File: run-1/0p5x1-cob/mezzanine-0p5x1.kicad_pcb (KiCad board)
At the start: 2 copper layers, 14 x 16 mm, 11 parts

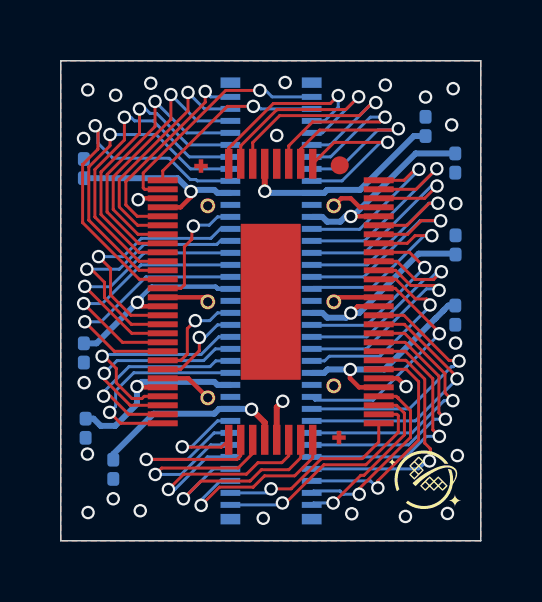
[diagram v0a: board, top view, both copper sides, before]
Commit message: Tweaks
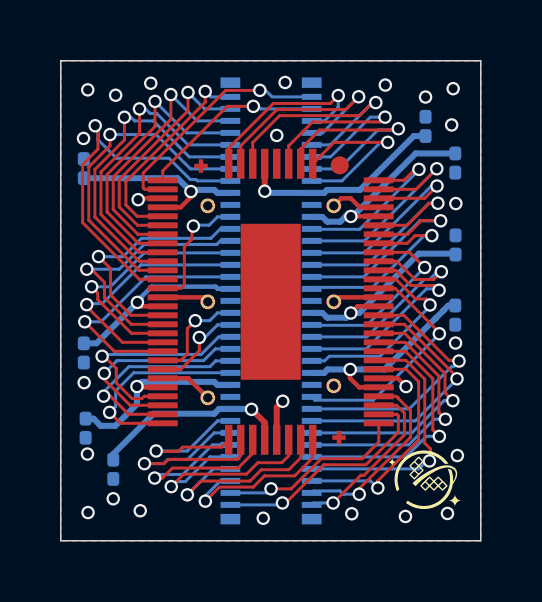
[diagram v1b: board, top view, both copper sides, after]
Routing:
- net /an_0: track 3.62 -> 5.48 mm
